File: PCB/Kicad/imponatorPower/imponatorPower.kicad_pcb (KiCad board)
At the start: 2 copper layers, 60.2 x 31.4 mm, 29 parts, among them J1 UJ20-C-H-G-SMT-1-P16-TR, J2 Conn_01x02, U1 BQ25172DSGR, U2 MP28164GD-Z

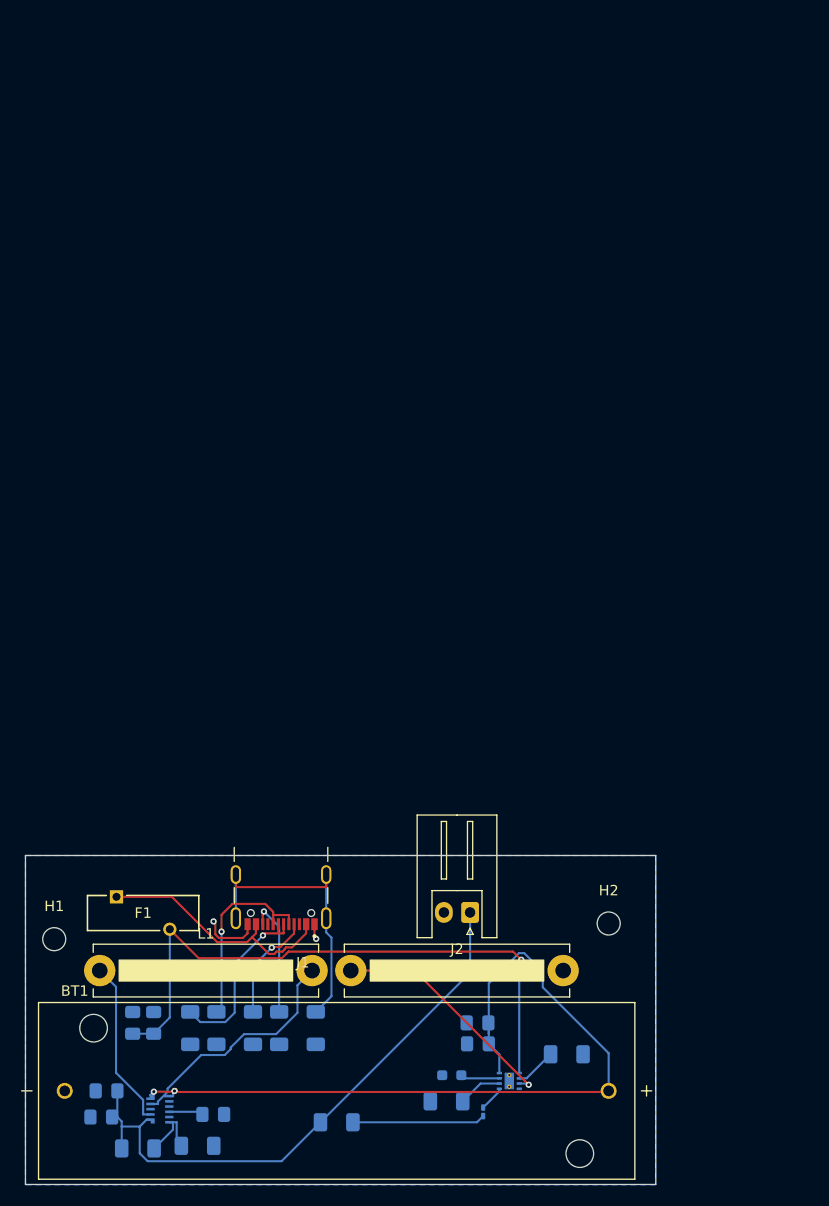
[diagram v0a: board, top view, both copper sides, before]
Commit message: Finished the second iteration of the imponatorPower project
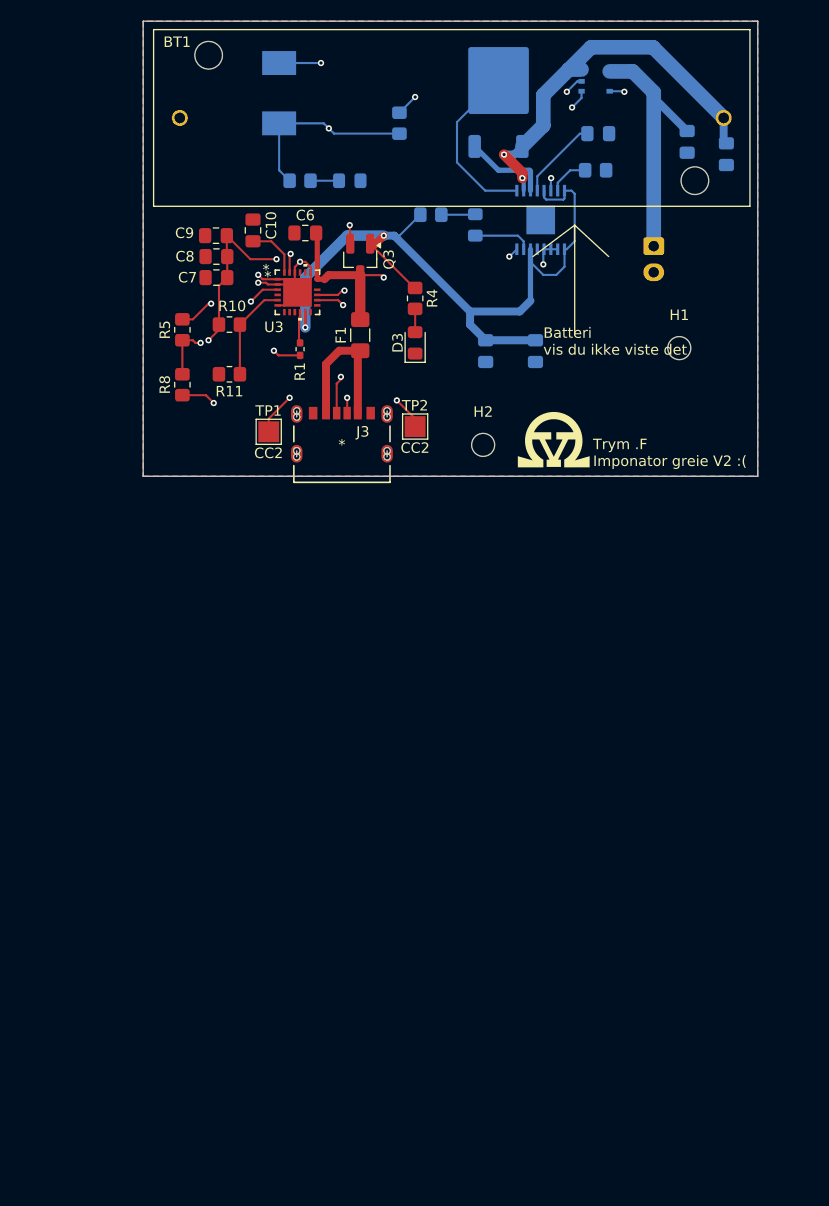
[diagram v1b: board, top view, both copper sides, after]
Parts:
- removed J1: UJ20-C-H-G-SMT-1-P16-TR, Imported:SAMESKY_UJ20-C-H-G-SMT-1-P16-TR
- removed R12: 100K, Resistor_SMD:R_1206_3216Metric_Pad1.30x1.75mm_HandSolder
- removed R2: 56K, Resistor_SMD:R_1206_3216Metric_Pad1.30x1.75mm_HandSolder
- added C10: 1uF, Capacitor_SMD:C_0805_2012Metric_Pad1.18x1.45mm_HandSolder, F.Cu at (109.0, 80.2)
- added C8: 100nF, Capacitor_SMD:C_0805_2012Metric_Pad1.18x1.45mm_HandSolder, F.Cu at (105.5, 82.8)
- added C9: 100nF, Capacitor_SMD:C_0805_2012Metric_Pad1.18x1.45mm_HandSolder, F.Cu at (105.5, 80.8)
- added D2: LED, LED_SMD:LED_0805_2012Metric_Pad1.15x1.40mm_HandSolder, B.Cu at (130.2, 79.7)
- added D3: LED, LED_SMD:LED_0805_2012Metric_Pad1.15x1.40mm_HandSolder, F.Cu at (124.5, 91.0)
- added G***: LOGO, LOGO, F.Cu at (137.8, 100.2)
- added J3: USB-C, Imported:2171750001_MOL, F.Cu at (117.5, 100.8)
- added Q1: MJD210G, Package_TO_SOT_SMD:TO-252-2, B.Cu at (132.5, 67.2)
- added Q3: PMOS, Package_TO_SOT_SMD:SOT-23_Handsoldering, F.Cu at (119.2, 83.0)
- added TP1: CC2, TestPoint:TestPoint_Pad_2.0x2.0mm, F.Cu at (110.5, 99.5)
- added TP2: CC2, TestPoint:TestPoint_Pad_2.0x2.0mm, F.Cu at (124.5, 99.0)
- added U3: CYPD, Imported:QFN24_CYPD3177_INF-L, F.Cu at (113.2, 86.2)
- C1, C2: value 100nF -> 10uF
- C3: value 1uF -> 1.5nF
- C4, C5: value 22uF -> 10uF
- C6: value 22uF -> 1uF; moved to F.Cu
- C7: moved to F.Cu
- D1: footprint LED_SMD:LED_0201_0603Metric_Pad0.64x0.40mm_HandSolder -> LED_SMD:LED_0805_2012Metric_Pad1.15x1.40mm_HandSolder
- F1: value MF-R075 -> Polyswitch; footprint Imported:FUS_MF-R075_BRN -> Fuse:Fuse_1206_3216Metric_Pad1.42x1.75mm_HandSolder
- J2: moved to B.Cu
- L1: value 1uH -> 4.7uH; footprint Resistor_THT:R_Bare_Metal_Element_L21.3mm_W4.8mm_P20.30mm -> Imported:IND_PCC-M0754M_PAN-L; moved to B.Cu
- R1: value 1M -> 50k; footprint Resistor_SMD:R_1206_3216Metric_Pad1.30x1.75mm_HandSolder -> Resistor_SMD:R_0402_1005Metric_Pad0.72x0.64mm_HandSolder; moved to F.Cu
- R10: value 10K -> 5.1k; footprint Resistor_SMD:R_1206_3216Metric_Pad1.30x1.75mm_HandSolder -> Resistor_SMD:R_0805_2012Metric_Pad1.20x1.40mm_HandSolder; moved to F.Cu
- R11: value 560K -> 2.4k; footprint Resistor_SMD:R_1206_3216Metric_Pad1.30x1.75mm_HandSolder -> Resistor_SMD:R_0805_2012Metric_Pad1.20x1.40mm_HandSolder; moved to F.Cu
- R3: value 56K -> 330; footprint Resistor_SMD:R_1206_3216Metric_Pad1.30x1.75mm_HandSolder -> Resistor_SMD:R_0805_2012Metric_Pad1.20x1.40mm_HandSolder
- R4: value 10K -> 330; footprint Resistor_SMD:R_1206_3216Metric_Pad1.30x1.75mm_HandSolder -> Resistor_SMD:R_0805_2012Metric_Pad1.20x1.40mm_HandSolder; moved to F.Cu
- R5: value 10K -> 47; footprint Resistor_SMD:R_1206_3216Metric_Pad1.30x1.75mm_HandSolder -> Resistor_SMD:R_0805_2012Metric_Pad1.20x1.40mm_HandSolder; moved to F.Cu
- R6: value 62K +- 1% -> 10K; footprint Resistor_SMD:R_0603_1608Metric_Pad0.98x0.95mm_HandSolder -> Resistor_SMD:R_0805_2012Metric_Pad1.20x1.40mm_HandSolder
- R7: value 1K -> 1.4k 1%; footprint Resistor_SMD:R_1206_3216Metric_Pad1.30x1.75mm_HandSolder -> Resistor_SMD:R_0805_2012Metric_Pad1.20x1.40mm_HandSolder
- R8: value 24K -> 100k; footprint Resistor_SMD:R_1206_3216Metric_Pad1.30x1.75mm_HandSolder -> Resistor_SMD:R_0805_2012Metric_Pad1.20x1.40mm_HandSolder; moved to F.Cu
- R9: value 103AT-2 -> 330; footprint Resistor_THT:R_Bare_Metal_Element_L21.3mm_W4.8mm_P20.30mm -> Resistor_SMD:R_0805_2012Metric_Pad1.20x1.40mm_HandSolder; moved to B.Cu
- U1: value BQ25172DSGR -> LTC4060EFE-PBF; footprint Imported:IC_BQ25172DSGR -> Imported:SSOP-16_FE_LIT-L
- U2: value MP28164GD-Z -> XC9141B50CMR-G; footprint Imported:QFN-11_MP28164_MNP -> Imported:SOT25_XC9141_TOR-L
- moved C4 109.7 mm to (154.2, 73.0), turned to -90 degrees
- moved U2 106.7 mm to (141.8, 66.0), turned to 0 degrees
- moved C5 106.3 mm to (150.5, 71.8), turned to -90 degrees
- moved BT1 93.6 mm to (128.0, 69.5)
- moved R6 91.1 mm to (123.0, 70.0), turned to 90 degrees
- moved D1 89.9 mm to (118.2, 75.5), turned to 180 degrees
- moved C3 87.8 mm to (142.0, 71.0), turned to 180 degrees
- moved L1 85.6 mm to (111.5, 67.1), turned to -90 degrees
- moved R7 84.5 mm to (141.8, 74.5), turned to 0 degrees
- moved U1 82.4 mm to (136.5, 79.2), turned to -90 degrees
- moved H1 82.2 mm to (149.8, 91.5)
- moved R3 81.1 mm to (113.5, 75.5), turned to 180 degrees
- moved C7 80.0 mm to (105.5, 84.8)
- moved C6 77.3 mm to (114.0, 80.5), turned to 0 degrees
- moved R10 76.9 mm to (106.8, 89.2), turned to 0 degrees
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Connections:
- BT1 pad P: Net-(U1-OUT) -> +Vbat
- C1 pad 1: +5V -> vdc_out
- C2 pad 1: +5V -> vdc_out
- C3 pad 2: Net-(U1-OUT) -> Net-(U1-TIMER)
- C4 pad 1: +5VL -> +Vbat
- C5 pad 1: +5VL -> +5Vout
- C6 pad 1: Net-(U1-OUT) -> GND
- C6 pad 2: GND -> +5VUSB
- C7 pad 1: Net-(U2-VCC) -> GND
- C7 pad 2: GND -> +3V3
- D1 pad 1: Net-(D1-K) -> GND
- F1 pad 2: +5V -> +5VUSB
- J2 pad 1: +5VL -> +5Vout
- L1 pad 1: Net-(U2-SW2) -> Net-(U2-LX)
- L1 pad 2: Net-(U2-SW1) -> +Vbat
- R1 pad 1: Net-(J1-SHIELD) -> +3V3
- R1 pad 2: GND -> Net-(U3-FLIP)
- R10 pad 1: Net-(D1-A) -> +3V3
- R10 pad 2: +5VL -> ISNK_coarse
- R11 pad 1: Net-(U2-FB) -> ISNK_coarse
- R11 pad 2: +5VL -> GND
- R3 pad 1: Net-(J1-CC1) -> Net-(D1-A)
- R3 pad 2: GND -> +Vbat
- R4 pad 1: Net-(J1-DN1) -> vdc_out
- R4 pad 2: GND -> Net-(D3-A)
- R5 pad 1: Net-(J1-DN2) -> Net-(Q3-G)
- R5 pad 2: GND -> EN
- R6 pad 1: GND -> +Vbat
- R6 pad 2: Net-(U1-VSET) -> Net-(U2-CE)
- R7 pad 1: GND -> Net-(U1-PROG)
- R7 pad 2: Net-(U1-ISET) -> GND
- R8 pad 1: Net-(U1-TMR) -> +5VUSB
- R8 pad 2: GND -> Net-(Q3-G)
- R9 pad 1: Net-(U1-TS) -> vdc_out
- R9 pad 2: GND -> Net-(D2-A)
- U1 pad 1: +5V -> Net-(Q1-B)
- U1 pad 10: (no net) -> GND
- U1 pad 11: (no net) -> GND
- U1 pad 2: Net-(U1-ISET) -> +Vbat
- U1 pad 3: Net-(U1-TS) -> Net-(Q1-E)
- U1 pad 4: GND -> Net-(U1-TIMER)
- U1 pad 5: Net-(D1-K) -> vdc_out
- U1 pad 6: Net-(U1-TMR) -> GND
- U1 pad 7: Net-(U1-VSET) -> Net-(U1-PROG)
- U1 pad 8: Net-(U1-OUT) -> vdc_out
- U1 pad 9: unconnected-(U1-EXP-Pad9) -> vdc_out
- U2 pad 1: Net-(U1-OUT) -> Net-(U2-CE)
- U2 pad 3: unconnected-(U2-PG-Pad3) -> +Vbat
- U2 pad 4: Net-(U2-VCC) -> +5Vout
- U2 pad 5: GND -> Net-(U2-LX)
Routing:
- net Net-(U1-OUT): track 76.8 -> 0.00 mm, vias 2 -> 0
- net vdc_out: track 0.00 -> 74.3 mm, vias 0 -> 2
- net +Vbat: track 0.00 -> 73.5 mm, vias 0 -> 3
- net +5V: track 59.1 -> 0.00 mm, vias 1 -> 0
- net +5VL: track 56.9 -> 0.00 mm
- net +5VUSB: track 0.00 -> 41.4 mm, vias 0 -> 2
- net Net-(U2-LX): track 0.00 -> 35.6 mm, vias 0 -> 2
- net Net-(J1-SHIELD): track 29.2 -> 0.00 mm
- net +3V3: track 0.00 -> 29.2 mm, vias 0 -> 4
- net Net-(Q3-G): track 0.00 -> 26.0 mm, vias 0 -> 2
- net Net-(J3-CC1): track 0.00 -> 25.8 mm, vias 0 -> 3
- net +5Vout: track 0.00 -> 24.8 mm
- net Net-(U2-SW1): track 22.7 -> 0.00 mm
- net Net-(U1-TS): track 22.5 -> 0.00 mm, vias 1 -> 0
- net Net-(J3-CC2): track 0.00 -> 21.2 mm, vias 0 -> 3
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- added copper zone on F.Cu, net GND
- added copper zone on In2.Cu, net GND
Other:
- board size 60.2 x 31.4 mm -> 58.8 x 43.5 mm
- copper layers 2 -> 4
- board text added: "Batteri vis du ikke viste det"
- board text added: "Trym .F Imponator greie V2 :("
